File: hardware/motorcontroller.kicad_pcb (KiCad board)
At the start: 2 copper layers, 99.7 x 88.9 mm, 97 parts, among them J1 UART Header, J10 Conn_01x04_Male, J11 Conn_02x03_Counter_Clockwise, J12 Conn_01x04_Male, J13 Conn_02x03_Counter_Clockwise, J14 Conn_01x04_Male, J15 Conn_02x03_Counter_Clockwise, J16 Screw_Terminal_01x02, J17 Screw_Terminal_01x02, J18 Conn_01x04_Male, J19 Screw_Terminal_01x02, J2 SPI Header, J20 Screw_Terminal_01x02, J21 Screw_Terminal_01x02, J22 Screw_Terminal_01x02, J23 Screw_Terminal_01x02, J3 I2C Header, J4 Conn_01x04_Male, J5 Conn_02x03_Counter_Clockwise, J6 Conn_01x04_Male, J7 Conn_02x03_Counter_Clockwise, J8 Conn_01x04_Male, J9 Conn_02x03_Counter_Clockwise, SW1 Reset, U1 ATmega1284P-AU, U2 TLV1117-33, U3 STP55NF06L, U4 STP55NF06L, U5 STP55NF06L, U6 STP55NF06L, U7 STP55NF06L, U8 STP55NF06L, Y1 16MHz

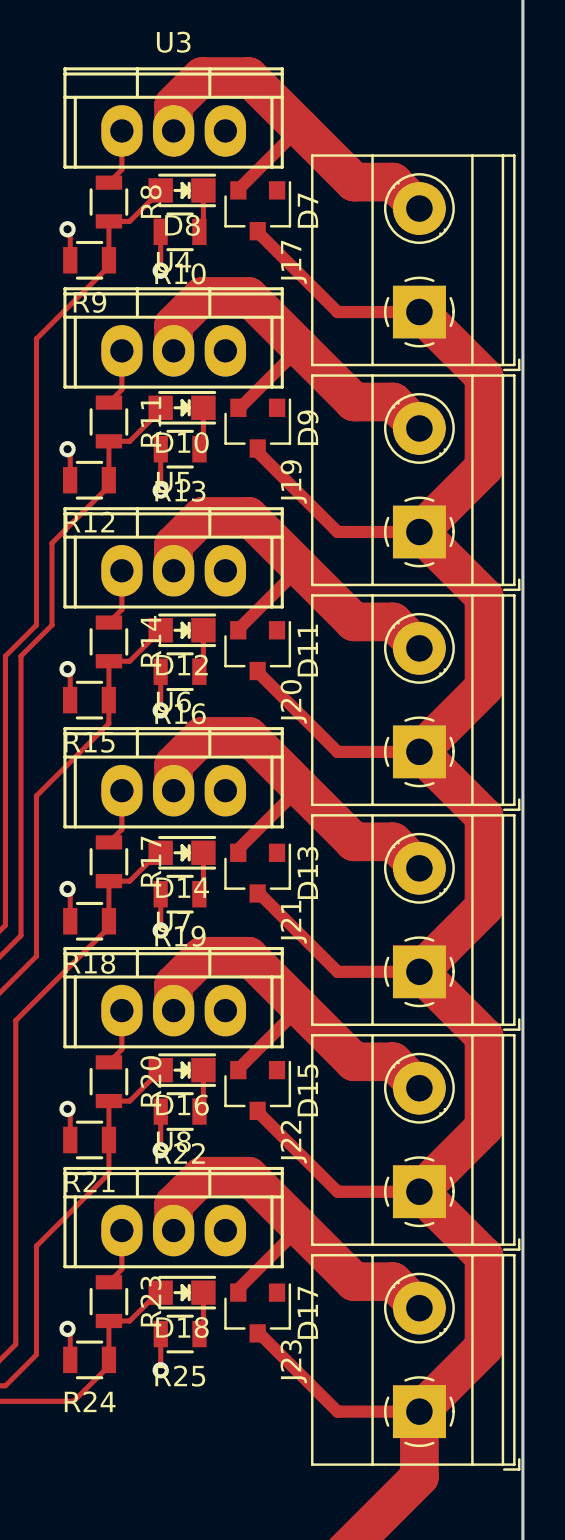
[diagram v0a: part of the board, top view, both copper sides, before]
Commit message: Cleanup
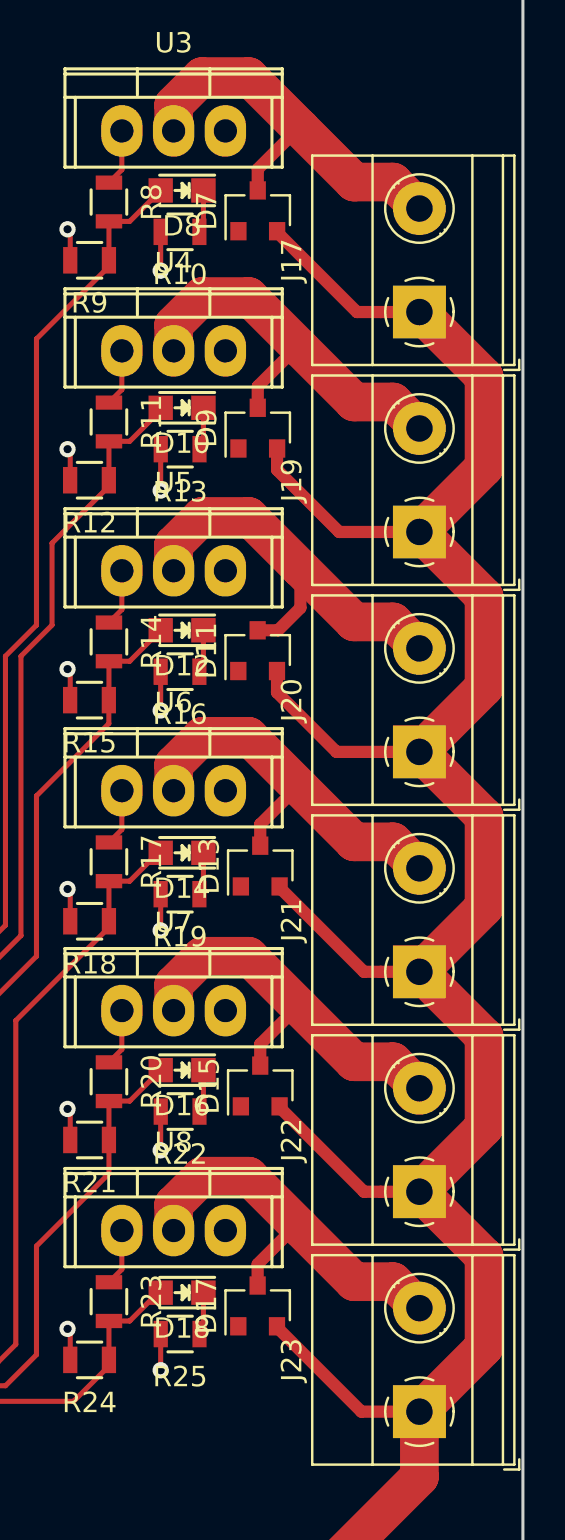
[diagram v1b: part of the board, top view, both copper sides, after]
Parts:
- moved D13 0.37 mm to (218.2, 81.2), turned to 90 degrees
- moved D17 0.35 mm to (218.1, 102.8), turned to 90 degrees
- moved D15 0.26 mm to (218.2, 92.0), turned to 90 degrees
- turned D11 to 90 degrees
- turned D7 to 90 degrees
- turned D9 to 90 degrees
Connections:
- A1 pad 9: Net-(A1-Pad9) -> (no net)
- A2 pad 9: Net-(A2-Pad9) -> (no net)
- A3 pad 9: Net-(A3-Pad9) -> (no net)
- A4 pad 9: Net-(A4-Pad9) -> (no net)
- A5 pad 9: Net-(A5-Pad9) -> (no net)
- A6 pad 9: Net-(A6-Pad9) -> (no net)
- D11 pad 1: Net-(D11-Pad1) -> (no net)
- D11 pad 2: Net-(D11-Pad2) -> +12V
- D11 pad 3: +12V -> Net-(D11-Pad3)
- D13 pad 1: Net-(D13-Pad1) -> (no net)
- D13 pad 2: Net-(D13-Pad2) -> +12V
- D13 pad 3: +12V -> Net-(D13-Pad3)
- D15 pad 1: Net-(D15-Pad1) -> (no net)
- D15 pad 2: Net-(D15-Pad2) -> +12V
- D15 pad 3: +12V -> Net-(D15-Pad3)
- D17 pad 1: Net-(D17-Pad1) -> (no net)
- D17 pad 2: Net-(D17-Pad2) -> +12V
- D17 pad 3: +12V -> Net-(D17-Pad3)
- D6 pad 2: Net-(D6-Pad2) -> (no net)
- D7 pad 1: Net-(D7-Pad1) -> (no net)
- D7 pad 2: Net-(D7-Pad2) -> +12V
- D7 pad 3: +12V -> Net-(D7-Pad3)
- D9 pad 1: Net-(D9-Pad1) -> (no net)
- D9 pad 2: Net-(D9-Pad2) -> +12V
- D9 pad 3: +12V -> Net-(D9-Pad3)
- J17 pad 2: Net-(D7-Pad2) -> Net-(D7-Pad3)
- J19 pad 2: Net-(D9-Pad2) -> Net-(D9-Pad3)
- J20 pad 2: Net-(D11-Pad2) -> Net-(D11-Pad3)
- J21 pad 2: Net-(D13-Pad2) -> Net-(D13-Pad3)
- J22 pad 2: Net-(D15-Pad2) -> Net-(D15-Pad3)
- J23 pad 2: Net-(D17-Pad2) -> Net-(D17-Pad3)
- U1 pad 11: Net-(U1-Pad11) -> (no net)
- U1 pad 42: Net-(U1-Pad42) -> (no net)
- U3 pad 2: Net-(D7-Pad2) -> Net-(D7-Pad3)
- U4 pad 2: Net-(D9-Pad2) -> Net-(D9-Pad3)
- U5 pad 2: Net-(D11-Pad2) -> Net-(D11-Pad3)
- U6 pad 2: Net-(D13-Pad2) -> Net-(D13-Pad3)
- U7 pad 2: Net-(D15-Pad2) -> Net-(D15-Pad3)
- U8 pad 2: Net-(D17-Pad2) -> Net-(D17-Pad3)
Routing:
- net Net-(D11-Pad3): track 0.00 -> 22.4 mm
- net Net-(D11-Pad2): track 22.1 -> 0.00 mm
- net Net-(D7-Pad2): track 20.9 -> 0.00 mm
- net Net-(D9-Pad2): track 20.8 -> 0.00 mm
- net Net-(D17-Pad2): track 20.8 -> 0.00 mm
- net Net-(D15-Pad2): track 20.8 -> 0.00 mm
- net Net-(D13-Pad2): track 20.8 -> 0.00 mm
- net Net-(D7-Pad3): track 0.00 -> 20.6 mm
- net Net-(D9-Pad3): track 0.00 -> 20.5 mm
- net Net-(D17-Pad3): track 0.00 -> 20.5 mm
- net Net-(D15-Pad3): track 0.00 -> 20.4 mm
- net Net-(D13-Pad3): track 0.00 -> 20.4 mm
- net +12V: track 454.7 -> 450.5 mm
- net Net-(U1-Pad11): track 0.54 -> 0.00 mm
- net (no net): track 0.00 -> 0.54 mm
